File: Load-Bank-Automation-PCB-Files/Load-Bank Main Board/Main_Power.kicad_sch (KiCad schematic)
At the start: 16 parts, among them J2 USB_C_Receptacle_USB2.0_14P, J3 Barrel_Jack_MountingPin, U3 USBLC6-2SC6, U7 AZ1117IH-3.3, U8 AZ1117IH-3.3

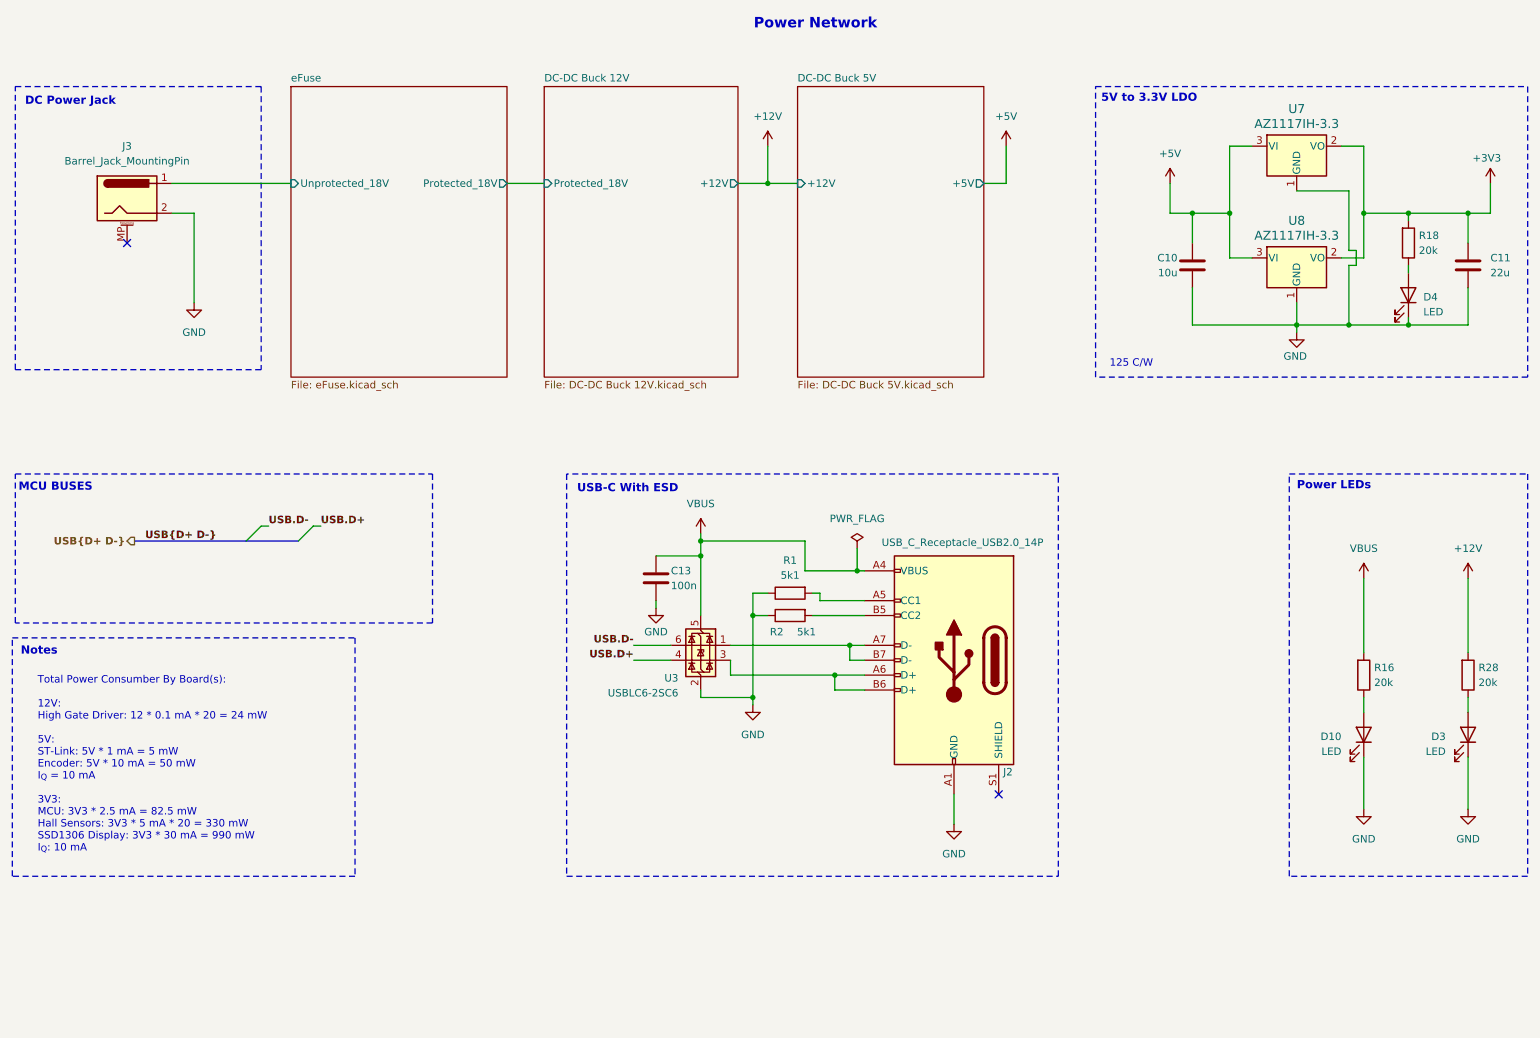
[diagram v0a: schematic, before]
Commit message: A
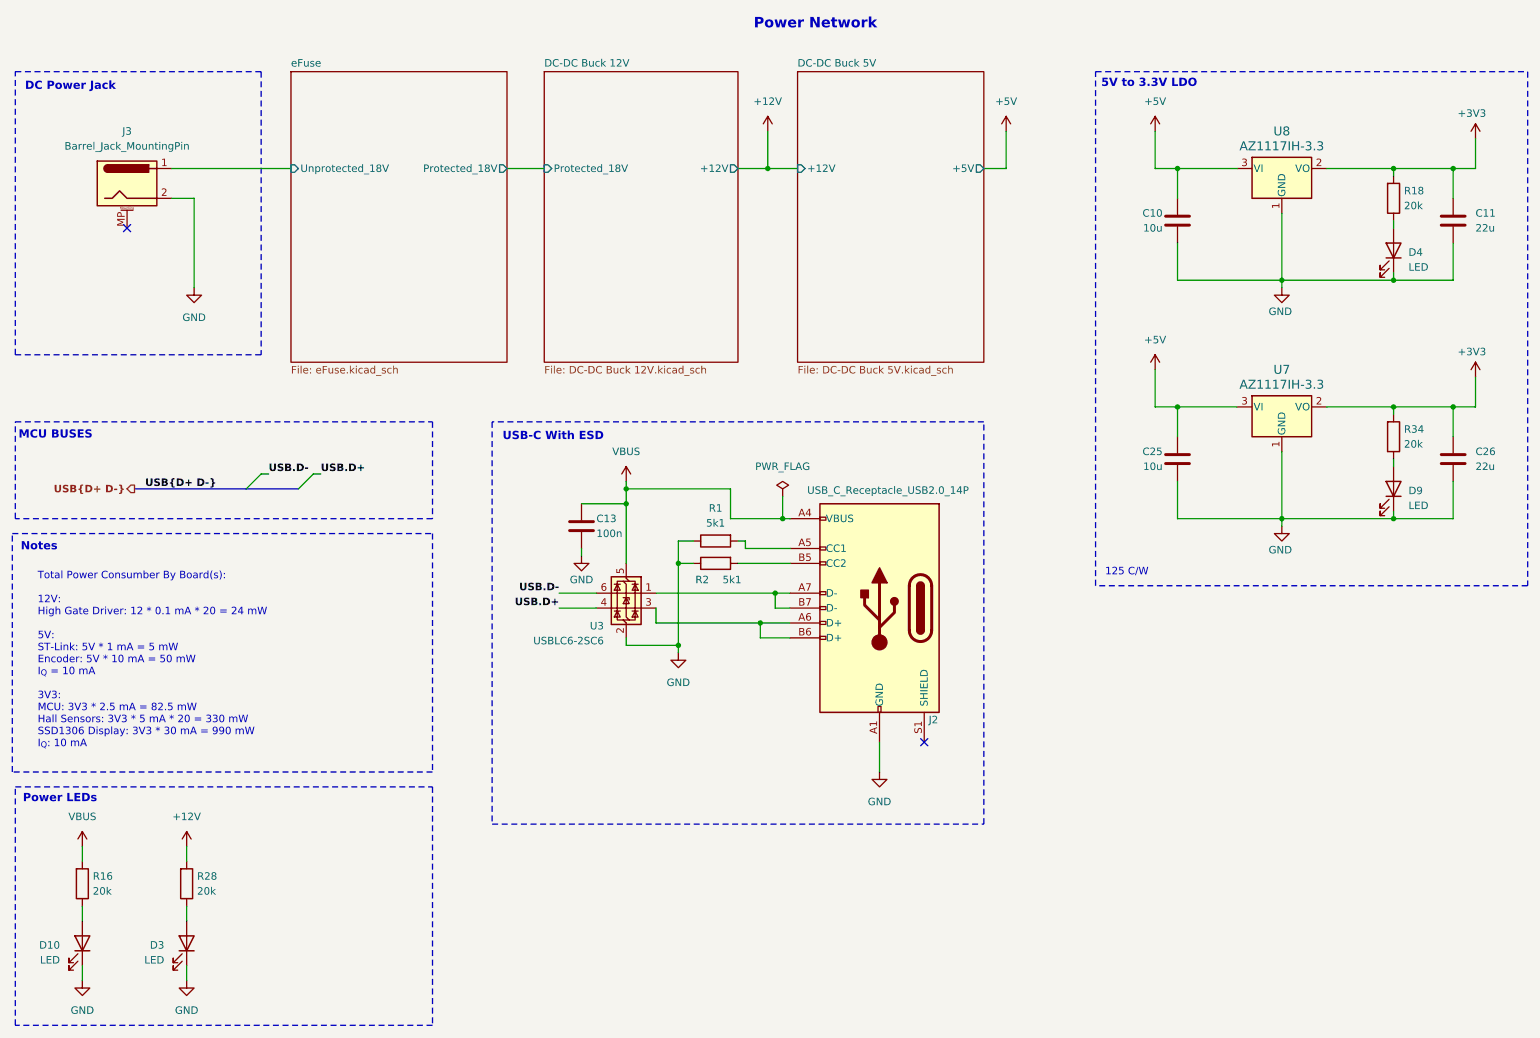
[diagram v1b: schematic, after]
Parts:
- added C25: 10u, Capacitor_SMD:C_1206_3216Metric_Pad1.33x1.80mm_HandSolder, symbol Device:C
- added C26: 22u, Capacitor_SMD:C_0805_2012Metric_Pad1.18x1.45mm_HandSolder, symbol Device:C
- added D9: LED, LED_SMD:LED_0603_1608Metric, symbol Device:LED
- added R34: 20k, Resistor_SMD:R_0603_1608Metric_Pad0.98x0.95mm_HandSolder, symbol Device:R
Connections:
- net +3V3: now also C26.1, R34.2
- net +5V: now also C25.1
- net GND: now also C25.2, C26.2, D9.1 (K)
- new net: D9.2 (A), R34.1
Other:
- moved on the sheet: C10, C11, C13, D10, D3, D4, J2, J3, R1, R16, R18, R2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
